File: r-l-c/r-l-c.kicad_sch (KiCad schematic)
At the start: 2 parts

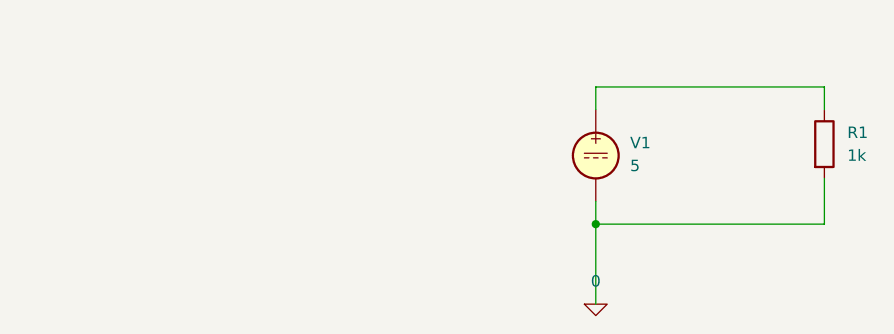
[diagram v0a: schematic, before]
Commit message: r-l-c simulation ok
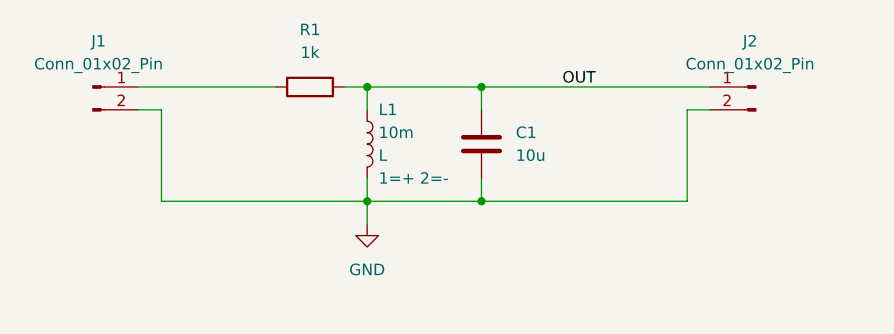
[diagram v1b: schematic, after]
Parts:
- removed V1: 5, symbol Simulation_SPICE:VDC
- added C1: 10u, symbol Device:C
- added J1, J2: Conn_01x02_Pin, symbol Connector:Conn_01x02_Pin
- added L1: 10m, symbol Device:L
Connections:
- net at R1.1: now also J1.1 (Pin_1)
- net 0 renamed OUT
- net OUT: now also C1.1, J2.1 (Pin_1), L1.1
- new net GND: C1.2, J1.2 (Pin_2), J2.2 (Pin_2), L1.2
